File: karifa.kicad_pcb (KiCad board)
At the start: 2 copper layers, 38.2 x 54.8 mm, 33 parts, among them J1 Conn_01x04, Q1 AO3401A, Q2 AO3401A, Q3 AO3401A, SW1 SW_DPST_x2, U1 STC8G1K08-SOP16

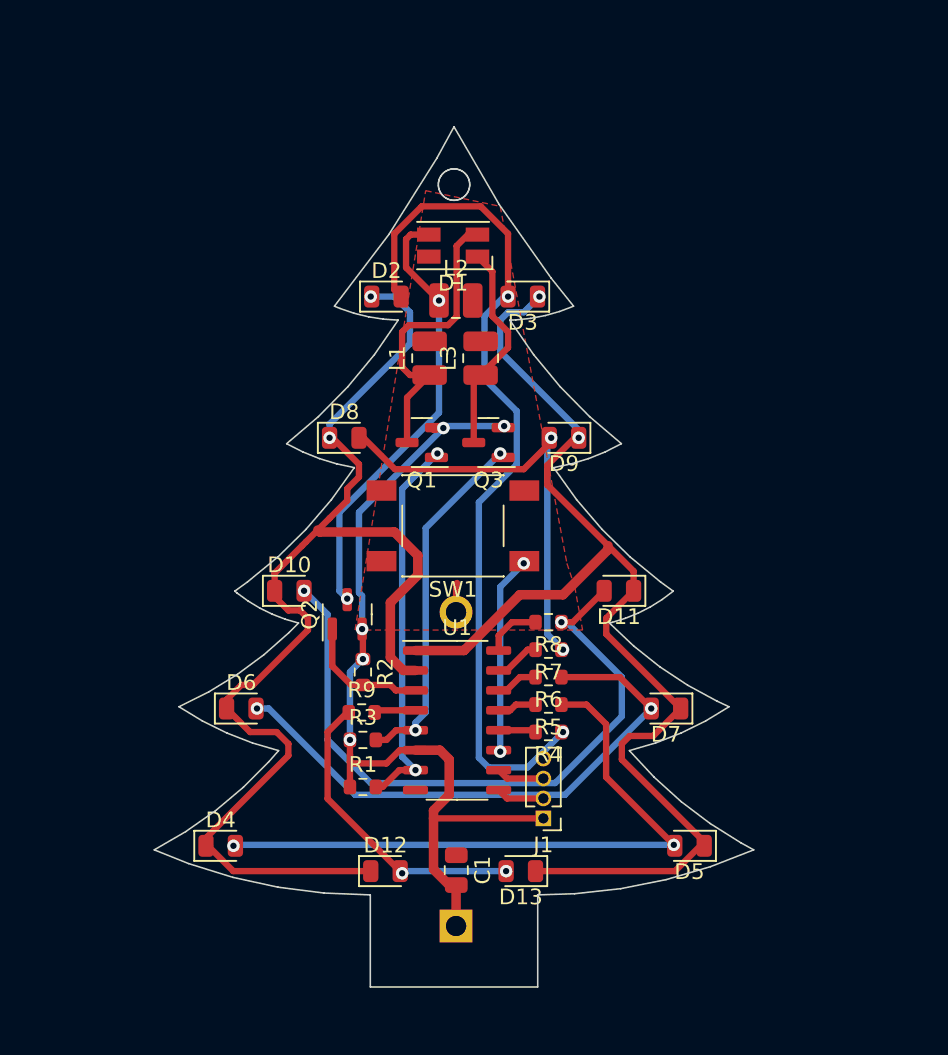
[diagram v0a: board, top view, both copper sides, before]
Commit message: nyakterv haladas
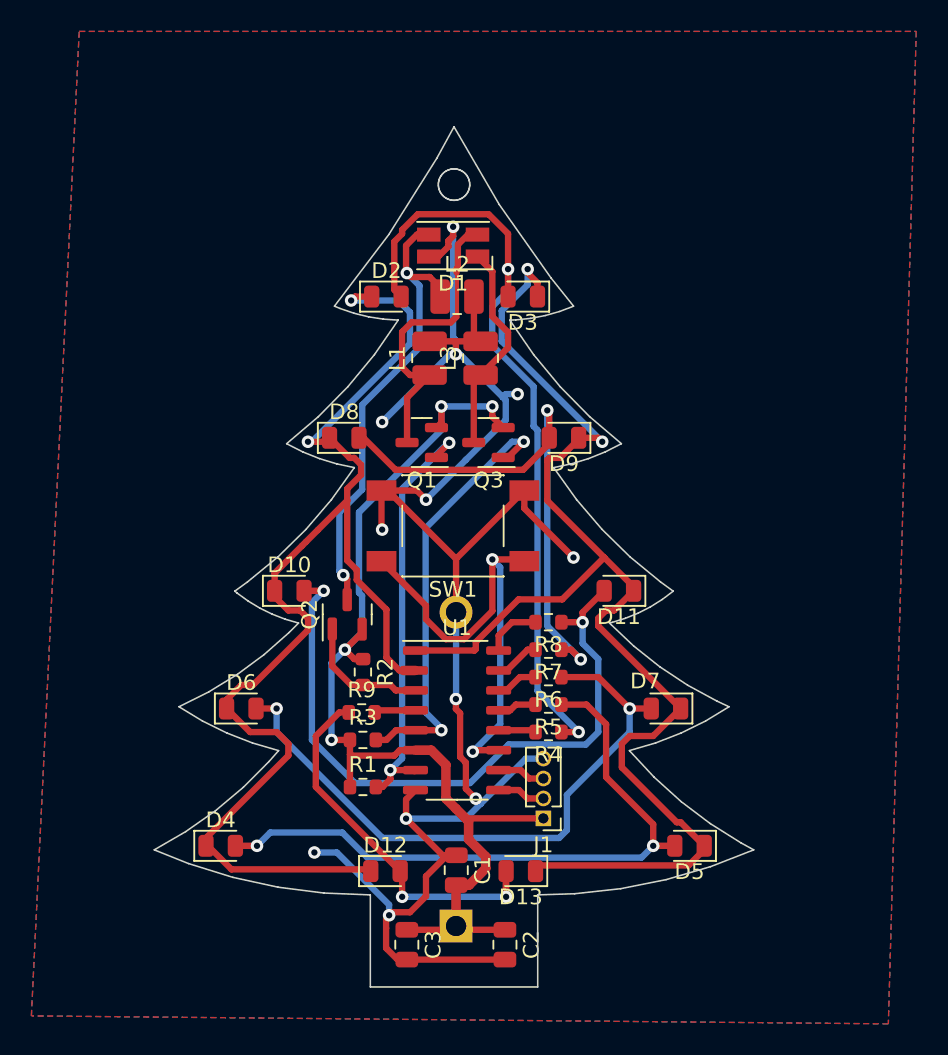
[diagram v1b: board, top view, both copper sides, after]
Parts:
- added C2: 10uF, Capacitor_SMD:C_0805_2012Metric, F.Cu at (133.3, 96.3)
- added C3: 10uF, Capacitor_SMD:C_0805_2012Metric, F.Cu at (127.0, 96.3)
- C1: value C -> 100nF
- R1, R2, R3: value R -> 100k
- R4, R5, R6, R7, R8, R9: value R -> 1k
- moved L2 0.26 mm to (130.2, 55.0)
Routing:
- net GND: track 1.89 -> 119.0 mm, vias 0 -> 12
- net Net-(SW1-Pad1): track 12.8 -> 30.6 mm
- net VCC: track 56.3 -> 69.6 mm, vias 5 -> 4
- net Net-(D8-Pad2): track 28.0 -> 34.1 mm
- net Net-(D12-Pad2): track 19.5 -> 25.3 mm
- net Net-(D2-Pad2): track 55.4 -> 49.6 mm
- net /MPX1: track 76.3 -> 81.9 mm
- net /P5.4: track 22.7 -> 28.0 mm
- net Net-(D6-Pad2): track 36.2 -> 40.3 mm
- net /MPX2: track 78.5 -> 81.5 mm
- net /P5.5: track 24.5 -> 27.0 mm
- net Net-(D1-Pad2): track 28.2 -> 30.3 mm
- net Net-(D4-Pad2): track 41.0 -> 41.7 mm
- added copper zone on B.Cu, net GND
